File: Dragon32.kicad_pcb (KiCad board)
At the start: 2 copper layers, 120.2 x 69.7 mm, 73 parts, among them IC1 74HCT273, IC10 74HCT32, IC11 74LS123N, IC12 LM1889N, IC15 CD4053, IC2 MC6847, IC3 74HCT00, IC4 74HCT20, IC5 74HCT86, IC6 74HCT393, IC7 74ALS74N, IC8 74HCT393, IC9 74HCT390, J1 Board Interconnect Male, J2 Video Output, U1 74AHC1G04, U2 MCP6281, Y1 4.433619MHz

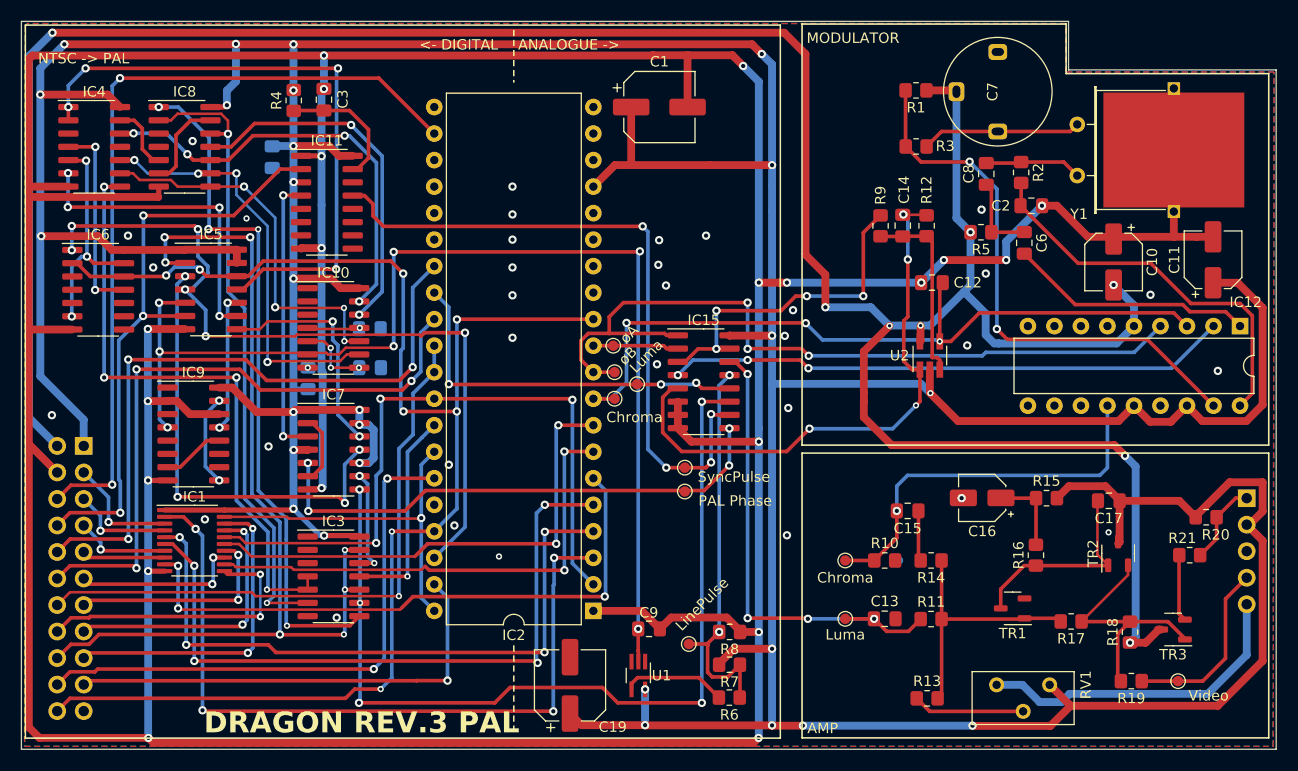
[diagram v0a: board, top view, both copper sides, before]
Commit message: reformat board
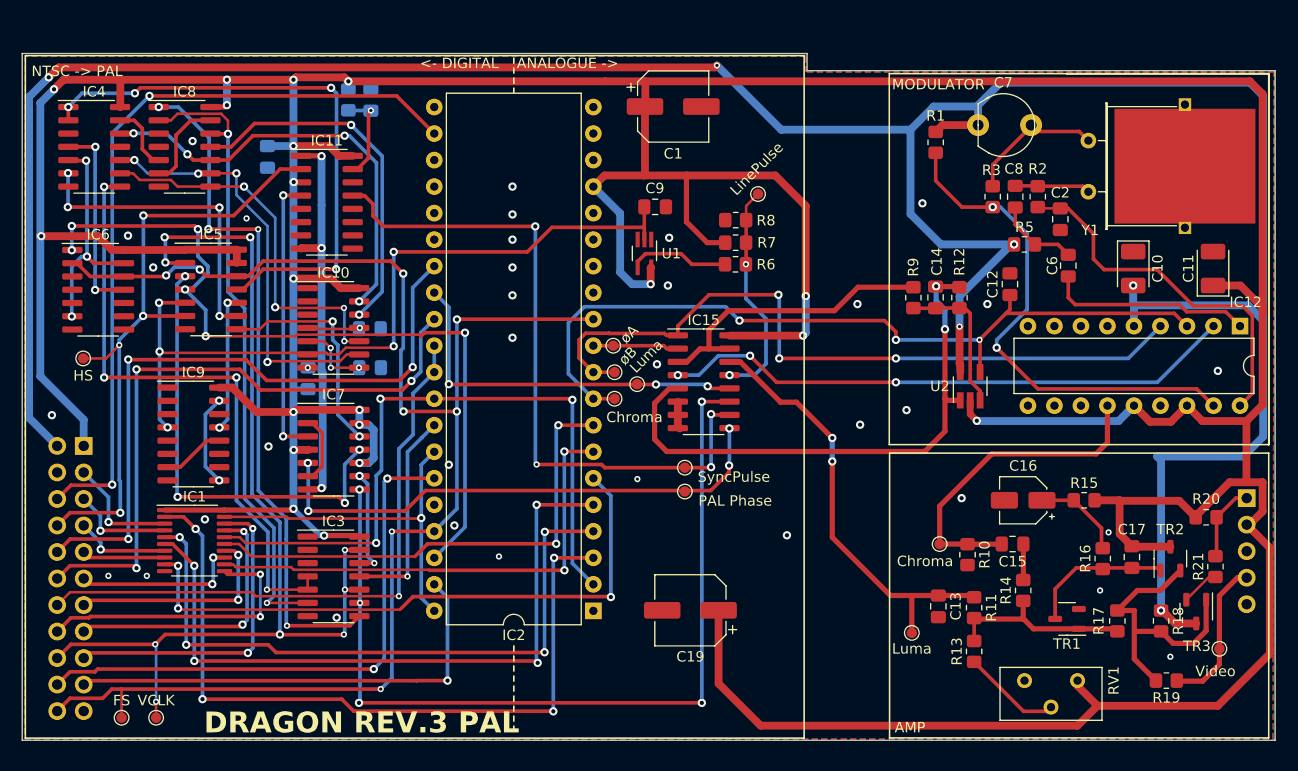
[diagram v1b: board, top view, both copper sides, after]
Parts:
- added TP11: TestPoint_FrameSync, TestPoint:TestPoint_Pad_D1.0mm, F.Cu at (93.5, 128.7)
- added TP12: TestPoint_LineSync, TestPoint:TestPoint_Pad_D1.0mm, F.Cu at (89.8, 94.2)
- added TP13: TestPoint_VCLK, TestPoint:TestPoint_Pad_D1.0mm, F.Cu at (96.8, 128.7)
- C10, C11: footprint Capacitor_SMD:CP_Elec_5x5.8 -> Capacitor_Tantalum_SMD:CP_EIA-3528-21_Kemet-B_Pad1.50x2.35mm_HandSolder
- C3, R4: moved to B.Cu
- C7: footprint Dragon:Trimmer-7.5mm -> Dragon:Trimmer_small
- TP5: value TestPoint_Composite -> TestPoint_Chroma
- moved TP10 43.6 mm to (154.4, 78.5)
- moved R6 41.5 mm to (152.3, 85.2)
- moved C9 40.4 mm to (144.6, 79.7)
- moved R7 40.4 mm to (152.3, 83.1)
- moved U1 40.4 mm to (143.6, 84.2)
- moved R8 39.5 mm to (152.3, 81.0), turned to 0 degrees
- moved C19 13.6 mm to (148.0, 118.4), turned to 180 degrees
- moved C15 10.5 mm to (178.8, 112.0)
- moved R14 9.27 mm to (179.8, 116.5), turned to 90 degrees
- moved TP5 9.18 mm to (171.8, 112.0)
- moved R3 8.77 mm to (176.9, 78.7), turned to -90 degrees
- moved R10 7.95 mm to (174.5, 113.0), turned to -90 degrees
- moved R9 7.56 mm to (169.3, 88.4)
- moved C14 7.56 mm to (171.4, 88.4)
- moved R12 7.56 mm to (173.7, 88.4)
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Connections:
- net Composite renamed Chroma
- net Net-(C15-Pad1) renamed /Chroma_a
- net Net-(IC15-Z0) renamed /MUX Zinput
- net Net-(TR1-B) renamed /Composite_a
- net Net-(TR2-E) renamed /Composite_b
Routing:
- net GND: track 511.7 -> 39.9 mm, vias 54 -> 38
- net /LINE PULSES: track 109.7 -> 74.8 mm, vias 7 -> 5
- net LINE PULSE: track 38.1 -> 21.3 mm
- net -5V: track 262.7 -> 278.2 mm, vias 8 -> 6
- net VCLK: track 91.1 -> 98.2 mm, vias 7 -> 9
- net /Composite_a: track 25.0 -> 18.1 mm
- net +5V: track 536.6 -> 543.2 mm, vias 27 -> 20
- net Chroma: track 37.7 -> 31.7 mm, vias 1 -> 0
- net Net-(TR1-C): track 19.7 -> 13.9 mm
- net CHB: track 73.4 -> 78.5 mm
- net phiB: track 76.0 -> 71.2 mm
- net Net-(IC4-Pad1): track 59.5 -> 55.1 mm
- net ChrOSC: track 53.0 -> 48.7 mm
- net DA0: track 77.4 -> 73.3 mm
- net MUX X: track 46.0 -> 41.9 mm, vias 4 -> 2
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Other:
- board size 120.2 x 69.7 mm -> 120 x 65.8 mm
